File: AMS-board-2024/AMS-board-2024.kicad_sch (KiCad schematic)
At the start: 45 parts, among them J1 XH_14pin_Side, J10 XH_14pin_Side, J11 XH_14pin_Side, J12 XH_14pin_Side, J13 XH_14pin_Side, J14 XH_14pin_Side, J15 XT30_2pin_Side, J16 XT30_2pin_Side, J17 XH_14pin_Side, J18 XH_14pin_Side, J19 XH_6pin_Side, J2 XH_14pin_Side, J20 XH_8pin_Side, J21 XH_2pin_Side, J22 PinHeader_02x05_P1.00mm, J23 XH_2pin_Side, J24 5077CR-16-SMC2-BK-TR, J3 XH_14pin_Side, J4 XH_14pin_Side, J5 XH_14pin_Side, J6 XH_14pin_Side, J7 XH_14pin_Side, J8 XH_14pin_Side, J9 XH_14pin_Side

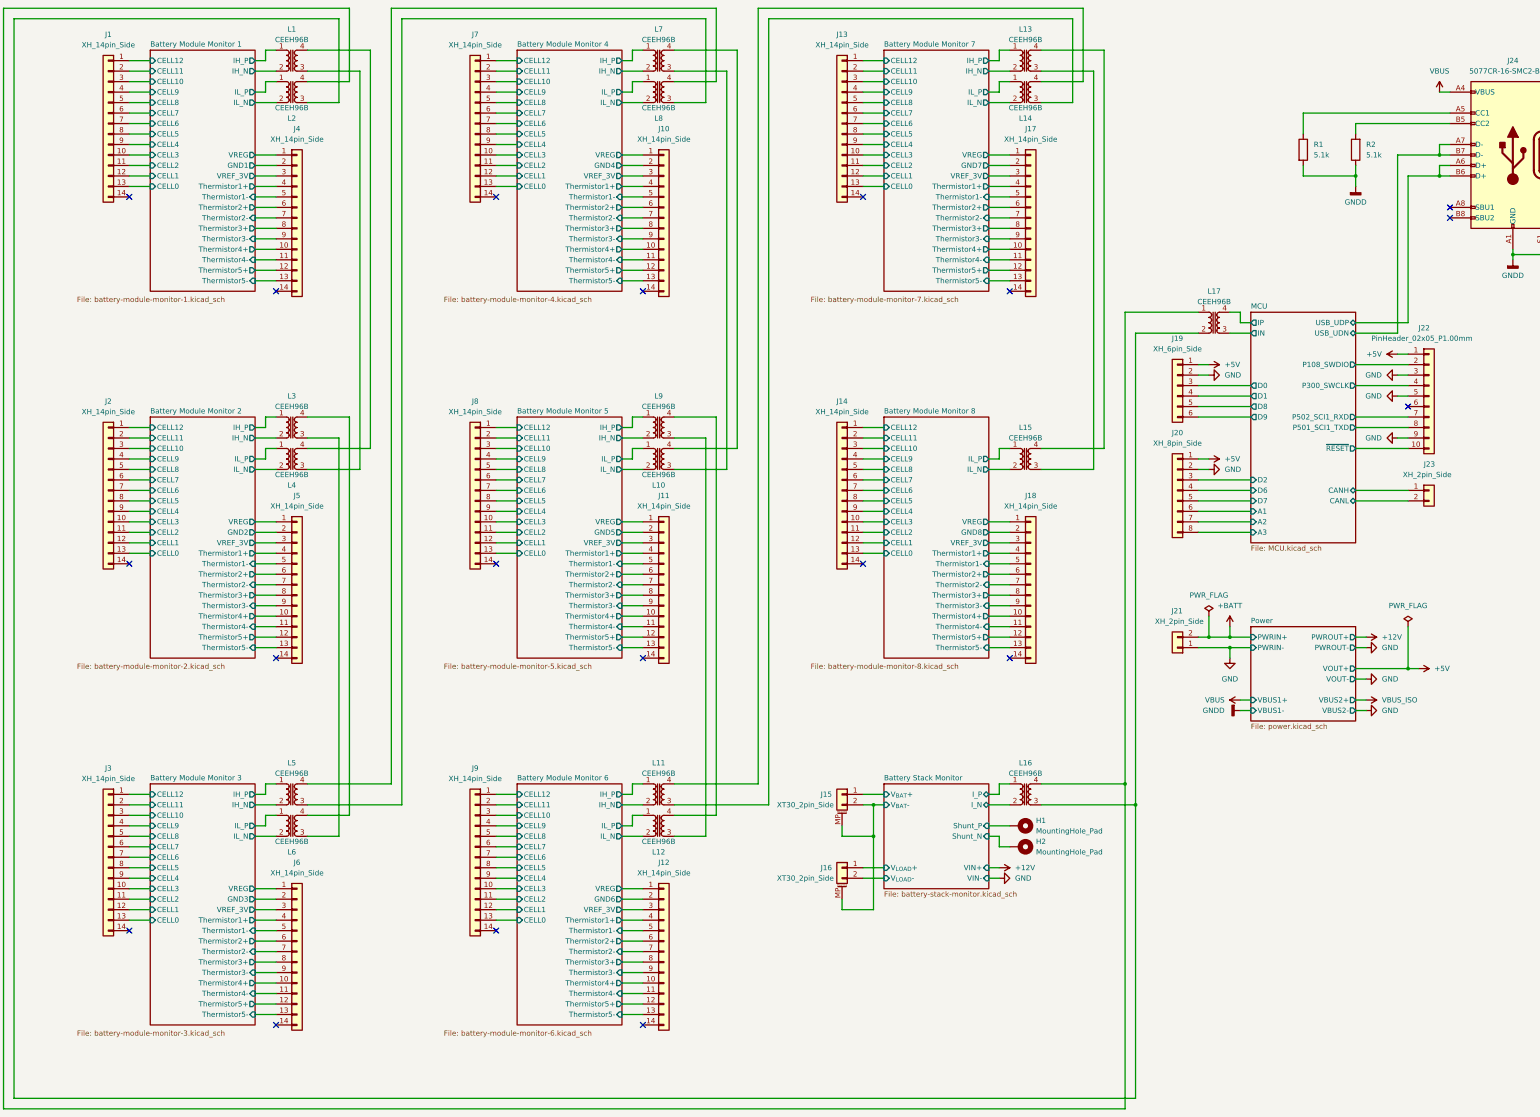
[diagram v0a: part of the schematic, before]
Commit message: コネクタをMX150Lに統一
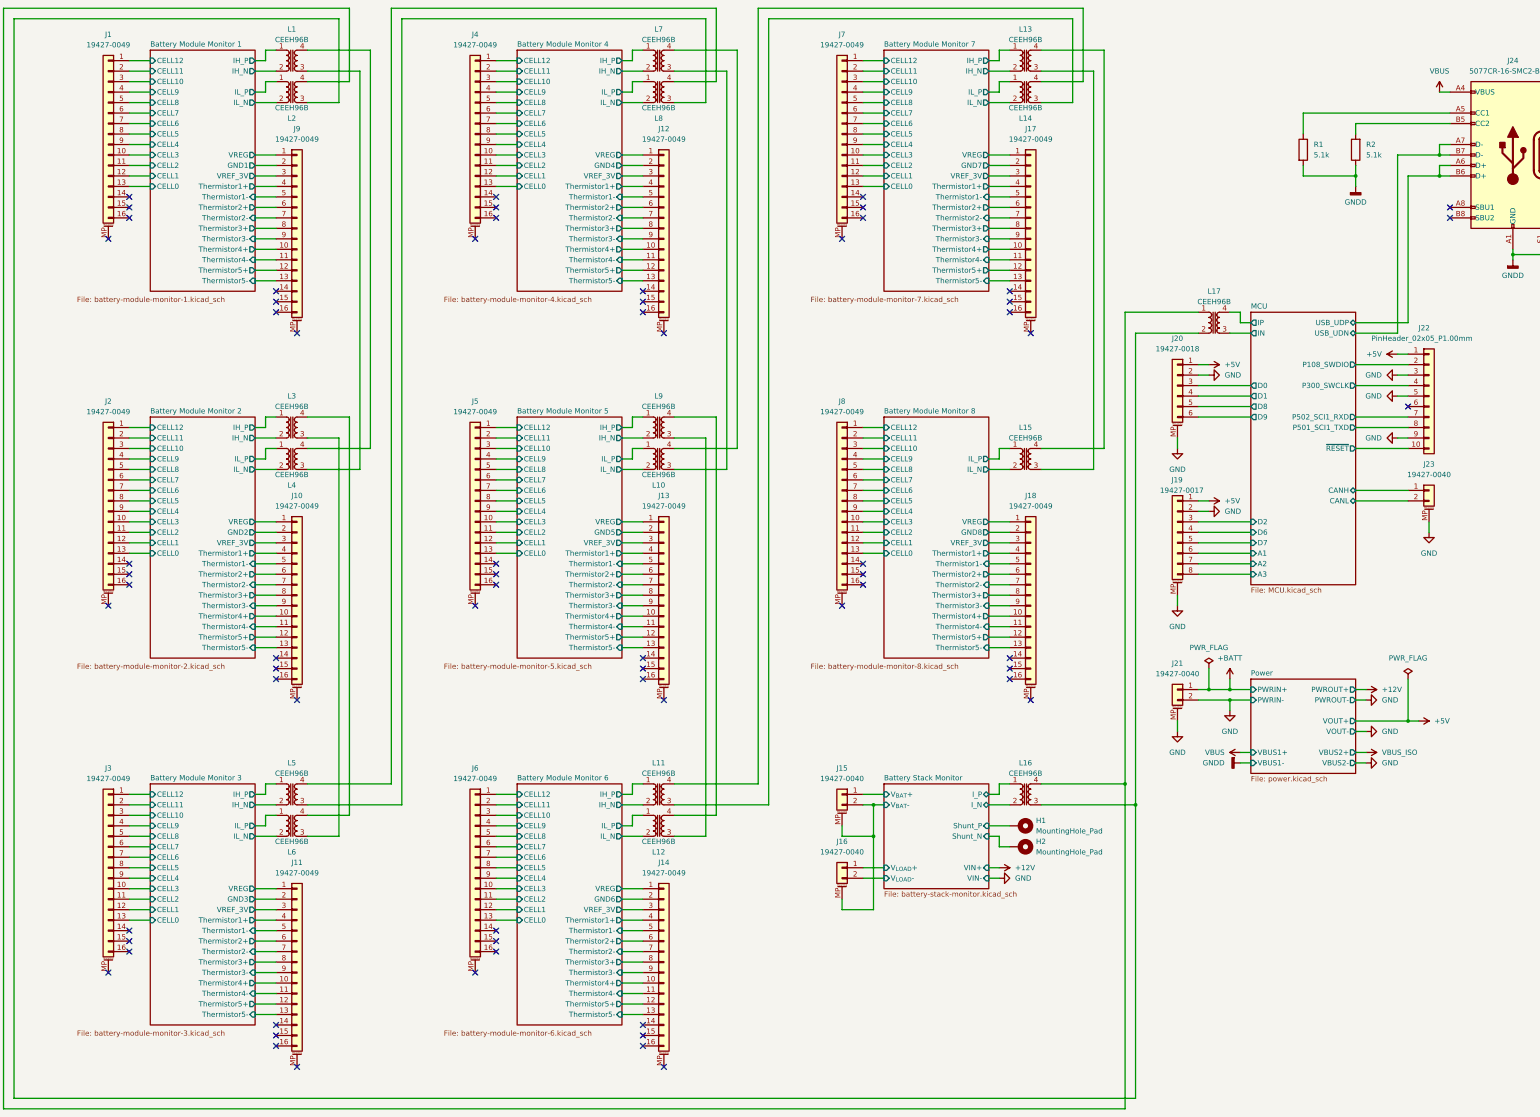
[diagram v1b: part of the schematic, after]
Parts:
- removed J1, J10, J11, J12, J13, J14, J17, J18, J2, J3, J4, J5, J6, J7, J8, J9: XH_14pin_Side, Connector_JST:JST_XH_S14B-XH-A_1x14_P2.50mm_Horizontal, symbol Connector_Generic:Conn_01x14
- removed J15, J16: XT30_2pin_Side, ProjectEV:Connector_XT30PW-M_1x02_P2.50mm_Horizontal, symbol ProjectEV:Connector_XT30PW-M
- removed J19: XH_6pin_Side, Connector_JST:JST_XH_S6B-XH-A_1x06_P2.50mm_Horizontal, symbol Connector_Generic:Conn_01x06
- removed J20: XH_8pin_Side, Connector_JST:JST_XH_S8B-XH-A_1x08_P2.50mm_Horizontal, symbol Connector_Generic:Conn_01x08
- removed J21, J23: XH_2pin_Side, Connector_JST:JST_XH_S2B-XH-A_1x02_P2.50mm_Horizontal, symbol Connector_Generic:Conn_01x02
- added J1, J10, J11, J12, J13, J14, J17, J18, J2, J3, J4, J5, J6, J7, J8, J9: 19427-0049, ProjectEV:Connector_MX150L_19427-0049, symbol ProjectEV:Connector_MX150L_19427-0049
- added J15, J16, J21, J23: 19427-0040, ProjectEV:Connector_MX150L_19427-0040, symbol ProjectEV:Connector_MX150L_19427-0040
- added J19: 19427-0017, ProjectEV:Connector_MX150L_19427-0017, symbol ProjectEV:Connector_MX150L_19427-0017
- added J20: 19427-0018, ProjectEV:Connector_MX150L_19427-0018, symbol ProjectEV:Connector_MX150L_19427-0018
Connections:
- net +5V: now also J19.1 (Pin_1), J20.1 (Pin_1)
- net +BATT: now also J21.1 (Pin_1)
- net Battery Module Monitor 1/CELL0: now also J1.13 (Pin_13)
- net Battery Module Monitor 1/CELL1: now also J1.12 (Pin_12)
- net Battery Module Monitor 1/CELL10: now also J1.3 (Pin_3)
- net Battery Module Monitor 1/CELL11: now also J1.2 (Pin_2)
- net Battery Module Monitor 1/CELL12: now also J1.1 (Pin_1)
- net Battery Module Monitor 1/CELL2: now also J1.11 (Pin_11)
- net Battery Module Monitor 1/CELL3: now also J1.10 (Pin_10)
- net Battery Module Monitor 1/CELL4: now also J1.9 (Pin_9)
- net Battery Module Monitor 1/CELL5: now also J1.8 (Pin_8)
- net Battery Module Monitor 1/CELL6: now also J1.7 (Pin_7)
- net Battery Module Monitor 1/CELL7: now also J1.6 (Pin_6)
- net Battery Module Monitor 1/CELL8: now also J1.5 (Pin_5)
- net Battery Module Monitor 1/CELL9: now also J1.4 (Pin_4)
- net Battery Module Monitor 1/GND1: now also J9.2 (Pin_2)
- net Battery Module Monitor 1/Thermistor1+: now also J9.4 (Pin_4)
- net Battery Module Monitor 1/Thermistor1-: now also J9.5 (Pin_5)
- net Battery Module Monitor 1/Thermistor2+: now also J9.6 (Pin_6)
- net Battery Module Monitor 1/Thermistor2-: now also J9.7 (Pin_7)
- net Battery Module Monitor 1/Thermistor3+: now also J9.8 (Pin_8)
- net Battery Module Monitor 1/Thermistor3-: now also J9.9 (Pin_9)
- net Battery Module Monitor 1/Thermistor4+: now also J9.10 (Pin_10)
- net Battery Module Monitor 1/Thermistor4-: now also J9.11 (Pin_11)
- net Battery Module Monitor 1/Thermistor5+: now also J9.12 (Pin_12)
- net Battery Module Monitor 1/Thermistor5-: now also J9.13 (Pin_13)
- net Battery Module Monitor 1/VREF_3V: now also J9.3 (Pin_3)
- net Battery Module Monitor 1/VREG: now also J9.1 (Pin_1)
- net Battery Module Monitor 2/CELL0: now also J2.13 (Pin_13)
- net Battery Module Monitor 2/CELL1: now also J2.12 (Pin_12)
- net Battery Module Monitor 2/CELL10: now also J2.3 (Pin_3)
- net Battery Module Monitor 2/CELL11: now also J2.2 (Pin_2)
- net Battery Module Monitor 2/CELL12: now also J2.1 (Pin_1)
- net Battery Module Monitor 2/CELL2: now also J2.11 (Pin_11)
- net Battery Module Monitor 2/CELL3: now also J2.10 (Pin_10)
- net Battery Module Monitor 2/CELL4: now also J2.9 (Pin_9)
- net Battery Module Monitor 2/CELL5: now also J2.8 (Pin_8)
- net Battery Module Monitor 2/CELL6: now also J2.7 (Pin_7)
- net Battery Module Monitor 2/CELL7: now also J2.6 (Pin_6)
- net Battery Module Monitor 2/CELL8: now also J2.5 (Pin_5)
- net Battery Module Monitor 2/CELL9: now also J2.4 (Pin_4)
- net Battery Module Monitor 2/GND2: now also J10.2 (Pin_2)
- net Battery Module Monitor 2/Thermistor1+: now also J10.4 (Pin_4)
- net Battery Module Monitor 2/Thermistor1-: now also J10.5 (Pin_5)
- net Battery Module Monitor 2/Thermistor2+: now also J10.6 (Pin_6)
- net Battery Module Monitor 2/Thermistor2-: now also J10.7 (Pin_7)
- net Battery Module Monitor 2/Thermistor3+: now also J10.8 (Pin_8)
- net Battery Module Monitor 2/Thermistor3-: now also J10.9 (Pin_9)
- net Battery Module Monitor 2/Thermistor4+: now also J10.10 (Pin_10)
- net Battery Module Monitor 2/Thermistor4-: now also J10.11 (Pin_11)
- net Battery Module Monitor 2/Thermistor5+: now also J10.12 (Pin_12)
- net Battery Module Monitor 2/Thermistor5-: now also J10.13 (Pin_13)
- net Battery Module Monitor 2/VREF_3V: now also J10.3 (Pin_3)
- net Battery Module Monitor 2/VREG: now also J10.1 (Pin_1)
- net Battery Module Monitor 3/CELL0: now also J3.13 (Pin_13)
- net Battery Module Monitor 3/CELL1: now also J3.12 (Pin_12)
- net Battery Module Monitor 3/CELL10: now also J3.3 (Pin_3)
- net Battery Module Monitor 3/CELL11: now also J3.2 (Pin_2)
- net Battery Module Monitor 3/CELL12: now also J3.1 (Pin_1)
- net Battery Module Monitor 3/CELL2: now also J3.11 (Pin_11)
- net Battery Module Monitor 3/CELL3: now also J3.10 (Pin_10)
- net Battery Module Monitor 3/CELL4: now also J3.9 (Pin_9)
- net Battery Module Monitor 3/CELL5: now also J3.8 (Pin_8)
- net Battery Module Monitor 3/CELL6: now also J3.7 (Pin_7)
- net Battery Module Monitor 3/CELL7: now also J3.6 (Pin_6)
- net Battery Module Monitor 3/CELL8: now also J3.5 (Pin_5)
- net Battery Module Monitor 3/CELL9: now also J3.4 (Pin_4)
- net Battery Module Monitor 3/GND3: now also J11.2 (Pin_2)
- net Battery Module Monitor 3/Thermistor1+: now also J11.4 (Pin_4)
- net Battery Module Monitor 3/Thermistor1-: now also J11.5 (Pin_5)
- net Battery Module Monitor 3/Thermistor2+: now also J11.6 (Pin_6)
- net Battery Module Monitor 3/Thermistor2-: now also J11.7 (Pin_7)
- net Battery Module Monitor 3/Thermistor3+: now also J11.8 (Pin_8)
- net Battery Module Monitor 3/Thermistor3-: now also J11.9 (Pin_9)
- net Battery Module Monitor 3/Thermistor4+: now also J11.10 (Pin_10)
- net Battery Module Monitor 3/Thermistor4-: now also J11.11 (Pin_11)
- net Battery Module Monitor 3/Thermistor5+: now also J11.12 (Pin_12)
- net Battery Module Monitor 3/Thermistor5-: now also J11.13 (Pin_13)
- net Battery Module Monitor 3/VREF_3V: now also J11.3 (Pin_3)
- net Battery Module Monitor 3/VREG: now also J11.1 (Pin_1)
- net Battery Module Monitor 4/CELL0: now also J4.13 (Pin_13)
- net Battery Module Monitor 4/CELL1: now also J4.12 (Pin_12)
- net Battery Module Monitor 4/CELL10: now also J4.3 (Pin_3)
- net Battery Module Monitor 4/CELL11: now also J4.2 (Pin_2)
- net Battery Module Monitor 4/CELL12: now also J4.1 (Pin_1)
- net Battery Module Monitor 4/CELL2: now also J4.11 (Pin_11)
- net Battery Module Monitor 4/CELL3: now also J4.10 (Pin_10)
- net Battery Module Monitor 4/CELL4: now also J4.9 (Pin_9)
- net Battery Module Monitor 4/CELL5: now also J4.8 (Pin_8)
- net Battery Module Monitor 4/CELL6: now also J4.7 (Pin_7)
- net Battery Module Monitor 4/CELL7: now also J4.6 (Pin_6)
- net Battery Module Monitor 4/CELL8: now also J4.5 (Pin_5)
- net Battery Module Monitor 4/CELL9: now also J4.4 (Pin_4)
- net Battery Module Monitor 4/GND4: now also J12.2 (Pin_2)
- net Battery Module Monitor 4/Thermistor1+: now also J12.4 (Pin_4)
- net Battery Module Monitor 4/Thermistor1-: now also J12.5 (Pin_5)
- net Battery Module Monitor 4/Thermistor2+: now also J12.6 (Pin_6)
- net Battery Module Monitor 4/Thermistor2-: now also J12.7 (Pin_7)
- net Battery Module Monitor 4/Thermistor3+: now also J12.8 (Pin_8)
- net Battery Module Monitor 4/Thermistor3-: now also J12.9 (Pin_9)
- net Battery Module Monitor 4/Thermistor4+: now also J12.10 (Pin_10)
- net Battery Module Monitor 4/Thermistor4-: now also J12.11 (Pin_11)
- net Battery Module Monitor 4/Thermistor5+: now also J12.12 (Pin_12)
- net Battery Module Monitor 4/Thermistor5-: now also J12.13 (Pin_13)
- net Battery Module Monitor 4/VREF_3V: now also J12.3 (Pin_3)
- net Battery Module Monitor 4/VREG: now also J12.1 (Pin_1)
- net Battery Module Monitor 5/CELL0: now also J5.13 (Pin_13)
- net Battery Module Monitor 5/CELL1: now also J5.12 (Pin_12)
- net Battery Module Monitor 5/CELL10: now also J5.3 (Pin_3)
- net Battery Module Monitor 5/CELL11: now also J5.2 (Pin_2)
- net Battery Module Monitor 5/CELL12: now also J5.1 (Pin_1)
- net Battery Module Monitor 5/CELL2: now also J5.11 (Pin_11)
- net Battery Module Monitor 5/CELL3: now also J5.10 (Pin_10)
- net Battery Module Monitor 5/CELL4: now also J5.9 (Pin_9)
- net Battery Module Monitor 5/CELL5: now also J5.8 (Pin_8)
- net Battery Module Monitor 5/CELL6: now also J5.7 (Pin_7)
- net Battery Module Monitor 5/CELL7: now also J5.6 (Pin_6)
- net Battery Module Monitor 5/CELL8: now also J5.5 (Pin_5)
- net Battery Module Monitor 5/CELL9: now also J5.4 (Pin_4)
- net Battery Module Monitor 5/GND5: now also J13.2 (Pin_2)
- net Battery Module Monitor 5/Thermistor1+: now also J13.4 (Pin_4)
- net Battery Module Monitor 5/Thermistor1-: now also J13.5 (Pin_5)
- net Battery Module Monitor 5/Thermistor2+: now also J13.6 (Pin_6)
- net Battery Module Monitor 5/Thermistor2-: now also J13.7 (Pin_7)
- net Battery Module Monitor 5/Thermistor3+: now also J13.8 (Pin_8)
- net Battery Module Monitor 5/Thermistor3-: now also J13.9 (Pin_9)
- net Battery Module Monitor 5/Thermistor4+: now also J13.10 (Pin_10)
- net Battery Module Monitor 5/Thermistor4-: now also J13.11 (Pin_11)
- net Battery Module Monitor 5/Thermistor5+: now also J13.12 (Pin_12)
- net Battery Module Monitor 5/Thermistor5-: now also J13.13 (Pin_13)
- net Battery Module Monitor 5/VREF_3V: now also J13.3 (Pin_3)
- net Battery Module Monitor 5/VREG: now also J13.1 (Pin_1)
- net Battery Module Monitor 6/CELL0: now also J6.13 (Pin_13)
- net Battery Module Monitor 6/CELL1: now also J6.12 (Pin_12)
- net Battery Module Monitor 6/CELL10: now also J6.3 (Pin_3)
- net Battery Module Monitor 6/CELL11: now also J6.2 (Pin_2)
- net Battery Module Monitor 6/CELL12: now also J6.1 (Pin_1)
- net Battery Module Monitor 6/CELL2: now also J6.11 (Pin_11)
- net Battery Module Monitor 6/CELL3: now also J6.10 (Pin_10)
- net Battery Module Monitor 6/CELL4: now also J6.9 (Pin_9)
- net Battery Module Monitor 6/CELL5: now also J6.8 (Pin_8)
- net Battery Module Monitor 6/CELL6: now also J6.7 (Pin_7)
- net Battery Module Monitor 6/CELL7: now also J6.6 (Pin_6)
- net Battery Module Monitor 6/CELL8: now also J6.5 (Pin_5)
- net Battery Module Monitor 6/CELL9: now also J6.4 (Pin_4)
- net Battery Module Monitor 6/GND6: now also J14.2 (Pin_2)
- net Battery Module Monitor 6/Thermistor1+: now also J14.4 (Pin_4)
- net Battery Module Monitor 6/Thermistor1-: now also J14.5 (Pin_5)
- net Battery Module Monitor 6/Thermistor2+: now also J14.6 (Pin_6)
- net Battery Module Monitor 6/Thermistor2-: now also J14.7 (Pin_7)
- net Battery Module Monitor 6/Thermistor3+: now also J14.8 (Pin_8)
- net Battery Module Monitor 6/Thermistor3-: now also J14.9 (Pin_9)
- net Battery Module Monitor 6/Thermistor4+: now also J14.10 (Pin_10)
- net Battery Module Monitor 6/Thermistor4-: now also J14.11 (Pin_11)
- net Battery Module Monitor 6/Thermistor5+: now also J14.12 (Pin_12)
- net Battery Module Monitor 6/Thermistor5-: now also J14.13 (Pin_13)
- net Battery Module Monitor 6/VREF_3V: now also J14.3 (Pin_3)
- net Battery Module Monitor 6/VREG: now also J14.1 (Pin_1)
- net Battery Module Monitor 7/CELL0: now also J7.13 (Pin_13)
- net Battery Module Monitor 7/CELL1: now also J7.12 (Pin_12)
- net Battery Module Monitor 7/CELL10: now also J7.3 (Pin_3)
- net Battery Module Monitor 7/CELL11: now also J7.2 (Pin_2)
- net Battery Module Monitor 7/CELL12: now also J7.1 (Pin_1)
- net Battery Module Monitor 7/CELL2: now also J7.11 (Pin_11)
- net Battery Module Monitor 7/CELL3: now also J7.10 (Pin_10)
- net Battery Module Monitor 7/CELL4: now also J7.9 (Pin_9)
- net Battery Module Monitor 7/CELL5: now also J7.8 (Pin_8)
- net Battery Module Monitor 7/CELL6: now also J7.7 (Pin_7)
- net Battery Module Monitor 7/CELL7: now also J7.6 (Pin_6)
- net Battery Module Monitor 7/CELL8: now also J7.5 (Pin_5)
- net Battery Module Monitor 7/CELL9: now also J7.4 (Pin_4)
- net Battery Module Monitor 7/GND7: now also J17.2 (Pin_2)
- net Battery Module Monitor 7/Thermistor1+: now also J17.4 (Pin_4)
- net Battery Module Monitor 7/Thermistor1-: now also J17.5 (Pin_5)
- net Battery Module Monitor 7/Thermistor2+: now also J17.6 (Pin_6)
- net Battery Module Monitor 7/Thermistor2-: now also J17.7 (Pin_7)
- net Battery Module Monitor 7/Thermistor3+: now also J17.8 (Pin_8)
- net Battery Module Monitor 7/Thermistor3-: now also J17.9 (Pin_9)
- net Battery Module Monitor 7/Thermistor4+: now also J17.10 (Pin_10)
- net Battery Module Monitor 7/Thermistor4-: now also J17.11 (Pin_11)
- net Battery Module Monitor 7/Thermistor5+: now also J17.12 (Pin_12)
- net Battery Module Monitor 7/Thermistor5-: now also J17.13 (Pin_13)
- net Battery Module Monitor 7/VREF_3V: now also J17.3 (Pin_3)
- net Battery Module Monitor 7/VREG: now also J17.1 (Pin_1)
- net Battery Module Monitor 8/CELL0: now also J8.13 (Pin_13)
- net Battery Module Monitor 8/CELL1: now also J8.12 (Pin_12)
- net Battery Module Monitor 8/CELL10: now also J8.3 (Pin_3)
- net Battery Module Monitor 8/CELL11: now also J8.2 (Pin_2)
- net Battery Module Monitor 8/CELL12: now also J8.1 (Pin_1)
- net Battery Module Monitor 8/CELL2: now also J8.11 (Pin_11)
- net Battery Module Monitor 8/CELL3: now also J8.10 (Pin_10)
- net Battery Module Monitor 8/CELL4: now also J8.9 (Pin_9)
- net Battery Module Monitor 8/CELL5: now also J8.8 (Pin_8)
- net Battery Module Monitor 8/CELL6: now also J8.7 (Pin_7)
- net Battery Module Monitor 8/CELL7: now also J8.6 (Pin_6)
- net Battery Module Monitor 8/CELL8: now also J8.5 (Pin_5)
- net Battery Module Monitor 8/CELL9: now also J8.4 (Pin_4)
- net Battery Module Monitor 8/GND8: now also J18.2 (Pin_2)
- net Battery Module Monitor 8/Thermistor1+: now also J18.4 (Pin_4)
- net Battery Module Monitor 8/Thermistor1-: now also J18.5 (Pin_5)
- net Battery Module Monitor 8/Thermistor2+: now also J18.6 (Pin_6)
- net Battery Module Monitor 8/Thermistor2-: now also J18.7 (Pin_7)
- net Battery Module Monitor 8/Thermistor3+: now also J18.8 (Pin_8)
- net Battery Module Monitor 8/Thermistor3-: now also J18.9 (Pin_9)
- net Battery Module Monitor 8/Thermistor4+: now also J18.10 (Pin_10)
- net Battery Module Monitor 8/Thermistor4-: now also J18.11 (Pin_11)
- net Battery Module Monitor 8/Thermistor5+: now also J18.12 (Pin_12)
- net Battery Module Monitor 8/Thermistor5-: now also J18.13 (Pin_13)
- net Battery Module Monitor 8/VREF_3V: now also J18.3 (Pin_3)
- net Battery Module Monitor 8/VREG: now also J18.1 (Pin_1)
- net Battery Stack Monitor/V_{BAT}+: now also J15.1 (Pin_1)
- net Battery Stack Monitor/V_{BAT}-: now also J15.2 (Pin_2), J15.MP (MountPin), J16.MP (MountPin)
- net Battery Stack Monitor/V_{LOAD}+: now also J16.1 (Pin_1)
- net Battery Stack Monitor/V_{LOAD}-: now also J16.2 (Pin_2)
- net GND: now also J19.2 (Pin_2), J19.MP (MountPin), J20.2 (Pin_2), J20.MP (MountPin), J21.2 (Pin_2), J21.MP (MountPin), J23.MP (MountPin)
- net MCU/A1: now also J19.6 (Pin_6)
- net MCU/A2: now also J19.7 (Pin_7)
- net MCU/A3: now also J19.8 (Pin_8)
- net MCU/CANH: now also J23.1 (Pin_1)
- net MCU/CANL: now also J23.2 (Pin_2)
- net MCU/D0: now also J20.3 (Pin_3)
- net MCU/D1: now also J20.4 (Pin_4)
- net MCU/D2: now also J19.3 (Pin_3)
- net MCU/D6: now also J19.4 (Pin_4)
- net MCU/D7: now also J19.5 (Pin_5)
- net MCU/D8: now also J20.5 (Pin_5)
- net MCU/D9: now also J20.6 (Pin_6)
- no-connect marks 19 -> 67
